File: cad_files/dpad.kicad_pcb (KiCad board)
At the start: 2 copper layers, 49 x 65 mm, 52 parts, among them J2 ftdi_conn, J3 Conn_01x02, J4 Conn_01x04, J5 Conn_01x04, SW1 SW_Push, SW2 SW_Push, SW3 SW_Push, SW4 SW_Push, U1 SY8401ABC, U2 AMS1117-3.3, U3 ESP32-WROOM-32U, U4 SWITCH_5-WAY_TACTIL_10X10, U5 Trans_CAN_SN65HVD230DR

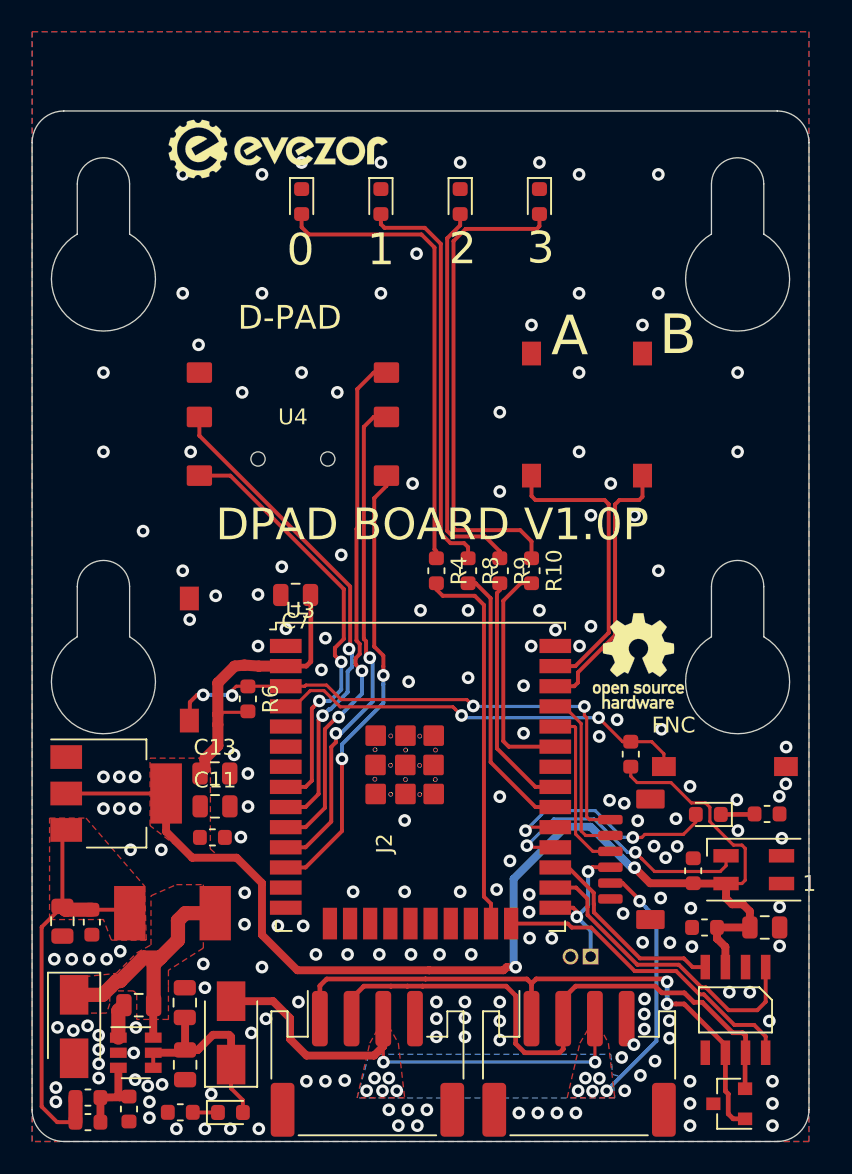
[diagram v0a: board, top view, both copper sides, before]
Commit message: Revert "add pics"
This reverts commit 85ade1bbc5e8a8a479c5a3c7b0c87c73afbe33f9.
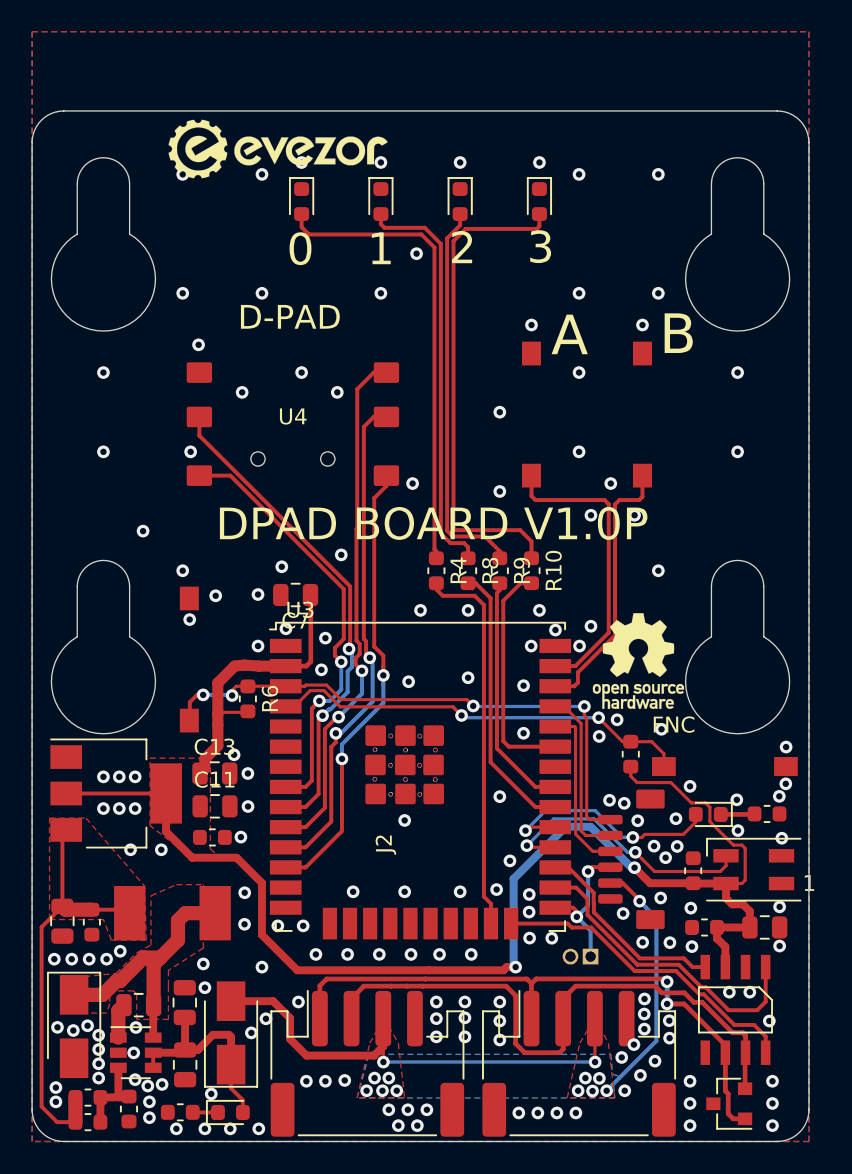
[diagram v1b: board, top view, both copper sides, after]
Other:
- outline, holes or cut-outs redrawn
- net class Default added: clearance 0.15, trace_width 0.25, via_dia 0.8, via_drill 0.4

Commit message: add pics
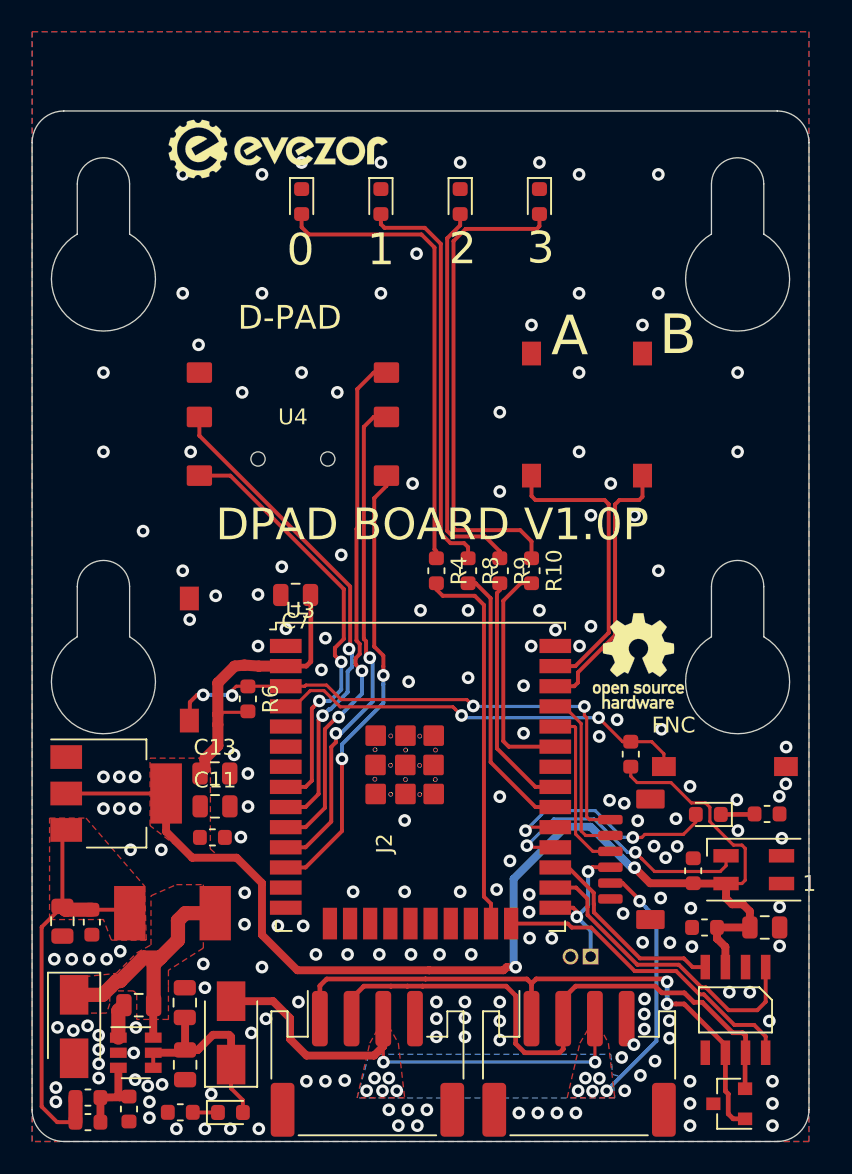
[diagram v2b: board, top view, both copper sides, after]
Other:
- outline, holes or cut-outs redrawn
- net class Default removed
